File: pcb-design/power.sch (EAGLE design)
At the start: 23 parts

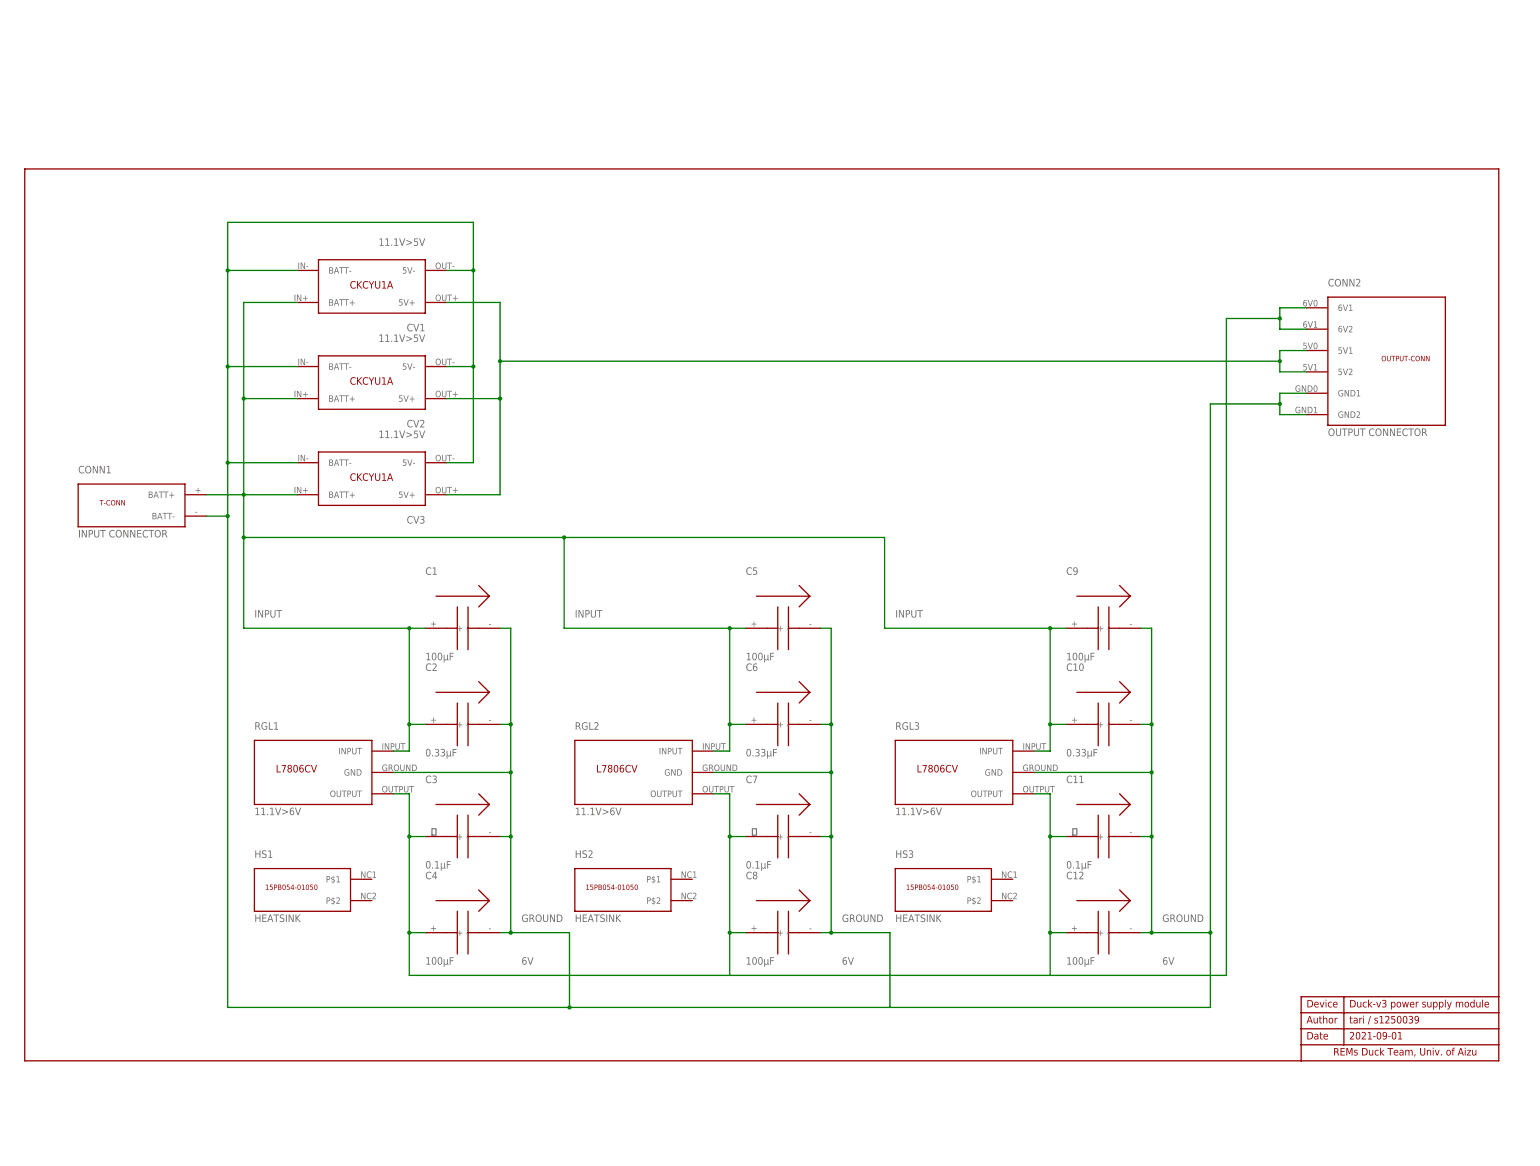
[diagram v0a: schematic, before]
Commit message: Before dinner
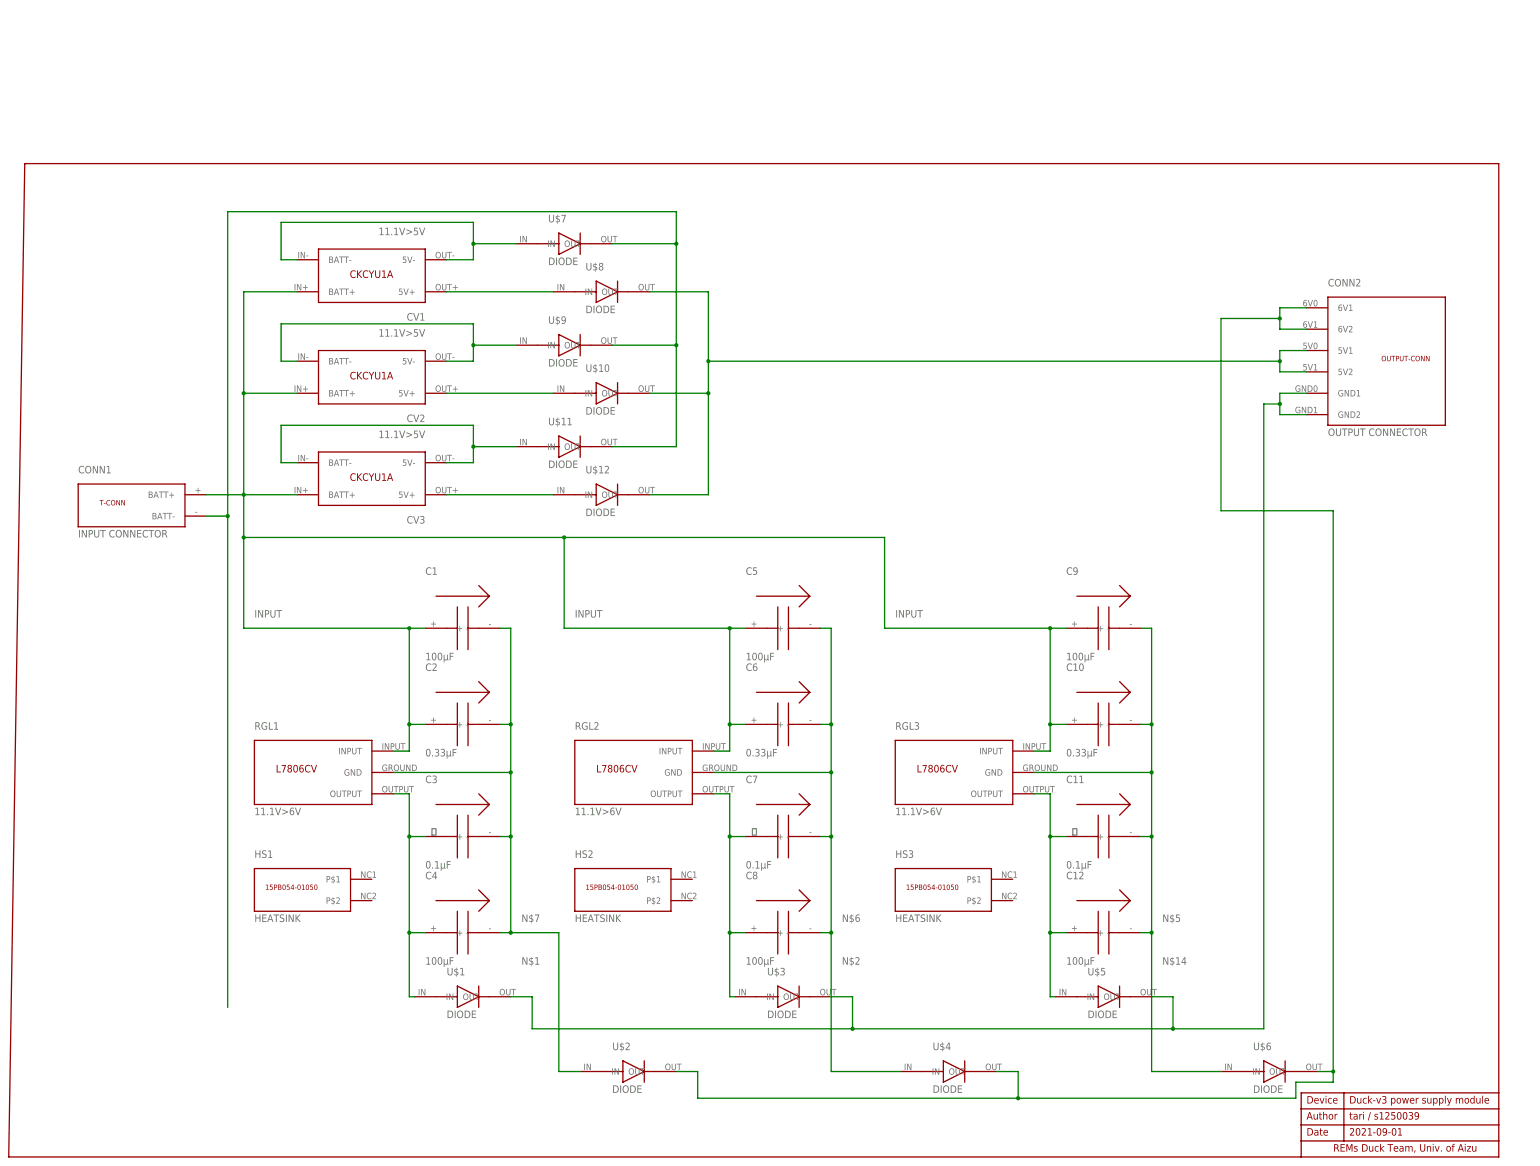
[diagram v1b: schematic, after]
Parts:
- added U$1, U$10, U$11, U$12, U$2, U$3, U$4, U$5, U$6, U$7, U$8, U$9: DIODE, library:DIODE
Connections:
- removed net 6V: C11.+, C12.+, C3.+, C4.+, C7.+, C8.+, CONN2.6V1, CONN2.6V2, RGL1.OUTPUT, RGL2.OUTPUT, RGL3.OUTPUT
- new net N$1: C3.+, C4.+, RGL1.OUTPUT, U$1.IN
- new net N$10: CONN2.5V1, CONN2.5V2, U$10.OUT, U$12.OUT, U$8.OUT
- new net N$11: CV1.5V-, CV1.BATT-, U$7.IN
- new net N$12: CV1.5V+, U$8.IN
- new net N$13: CV2.5V+, U$10.IN
- new net N$14: CONN2.6V1, CONN2.6V2, U$2.OUT, U$4.OUT, U$6.OUT
- new net N$2: C7.+, C8.+, RGL2.OUTPUT, U$3.IN
- new net N$3: CV3.5V-, CV3.BATT-, U$11.IN
- new net N$4: CONN2.GND1, CONN2.GND2, U$1.OUT, U$3.OUT, U$5.OUT
- new net N$5: C10.-, C11.-, C12.-, C9.-, RGL3.GND, U$6.IN
- new net N$6: C5.-, C6.-, C7.-, C8.-, RGL2.GND, U$4.IN
- new net N$7: C1.-, C2.-, C3.-, C4.-, RGL1.GND, U$2.IN
- new net N$8: C11.+, C12.+, RGL3.OUTPUT, U$5.IN
- new net N$9: CV2.5V-, CV2.BATT-, U$9.IN
- net 5V: now also U$12.IN; no longer CONN2.5V1, CONN2.5V2, CV1.5V+, CV2.5V+
- net GROUND: now also U$11.OUT, U$7.OUT, U$9.OUT; no longer C1.-, C10.-, C11.-, C12.-, C2.-, C3.-, C4.-, C5.-, C6.-, C7.-, C8.-, C9.-, CONN2.GND1, CONN2.GND2, CV1.5V-, CV1.BATT-, CV2.5V-, CV2.BATT-, CV3.5V-, CV3.BATT-, RGL1.GND, RGL2.GND, RGL3.GND
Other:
- moved on the sheet: CV1, CV2

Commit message: before lunch
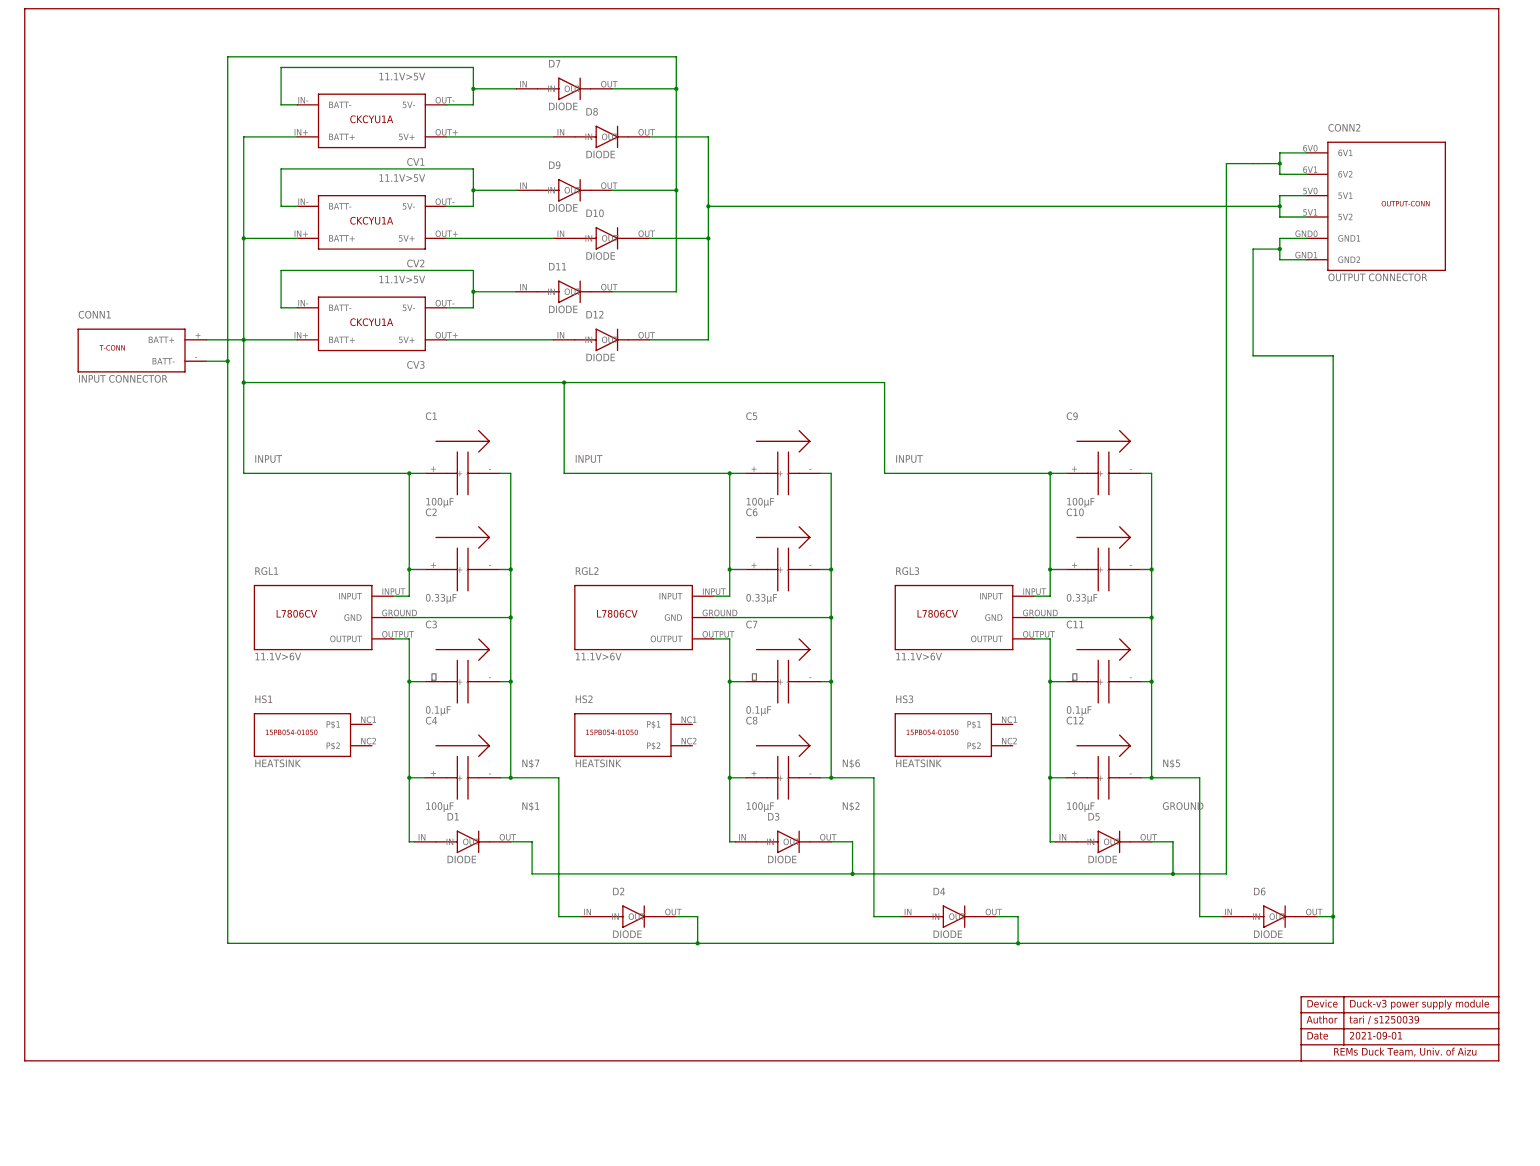
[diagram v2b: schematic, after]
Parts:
- removed U$1, U$10, U$11, U$12, U$2, U$3, U$4, U$5, U$6, U$7, U$8, U$9: DIODE, library:DIODE
- added D1, D10, D11, D12, D2, D3, D4, D5, D6, D7, D8, D9: DIODE, library:DIODE
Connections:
- removed net N$14: CONN2.6V1, CONN2.6V2, U$2.OUT, U$4.OUT, U$6.OUT
- net 5V: now also D12.IN; no longer U$12.IN
- net GROUND: now also CONN2.GND1, CONN2.GND2, D11.OUT, D2.OUT, D4.OUT, D6.OUT, D7.OUT, D9.OUT; no longer U$11.OUT, U$7.OUT, U$9.OUT
- net N$1: now also D1.IN; no longer U$1.IN
- net N$10: now also D10.OUT, D12.OUT, D8.OUT; no longer U$10.OUT, U$12.OUT, U$8.OUT
- net N$11: now also D7.IN; no longer U$7.IN
- net N$12: now also D8.IN; no longer U$8.IN
- net N$13: now also D10.IN; no longer U$10.IN
- net N$2: now also D3.IN; no longer U$3.IN
- net N$3: now also D11.IN; no longer U$11.IN
- net N$4: now also CONN2.6V1, CONN2.6V2, D1.OUT, D3.OUT, D5.OUT; no longer CONN2.GND1, CONN2.GND2, U$1.OUT, U$3.OUT, U$5.OUT
- net N$5: now also D6.IN; no longer U$6.IN
- net N$6: now also D4.IN; no longer U$4.IN
- net N$7: now also D2.IN; no longer U$2.IN
- net N$8: now also D5.IN; no longer U$5.IN
- net N$9: now also D9.IN; no longer U$9.IN
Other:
- moved on the sheet: C1, C10, C11, C12, C2, C3, C4, C5, C6, C7, C8, C9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
